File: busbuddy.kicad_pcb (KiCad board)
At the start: 2 copper layers, 77 x 54.5 mm, 48 parts, among them J201 GT-USB-7010ASV, J301 Conn_01x05_Pin, J302 Conn_01x10_Pin, J401 FH12A-24S-0.5SH(55), Q201 S8050, Q202 S8050, Q401 Q_NMOS_GSD, SW301 TS-1088R-02026, SW302 TS-1088R-02026, U202 CP2104, U301 ESP-12F, U501 SPX3819M5-L-3-3

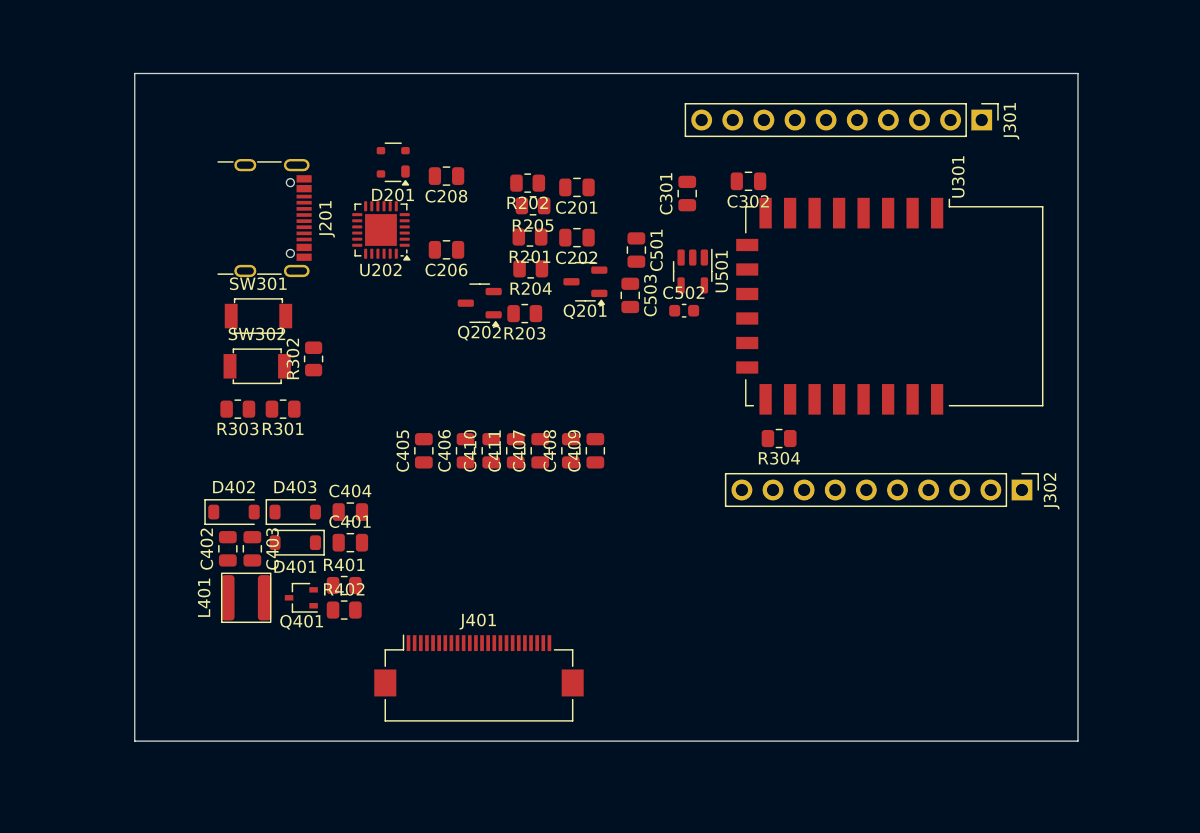
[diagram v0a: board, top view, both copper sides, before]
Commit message: Finish everything
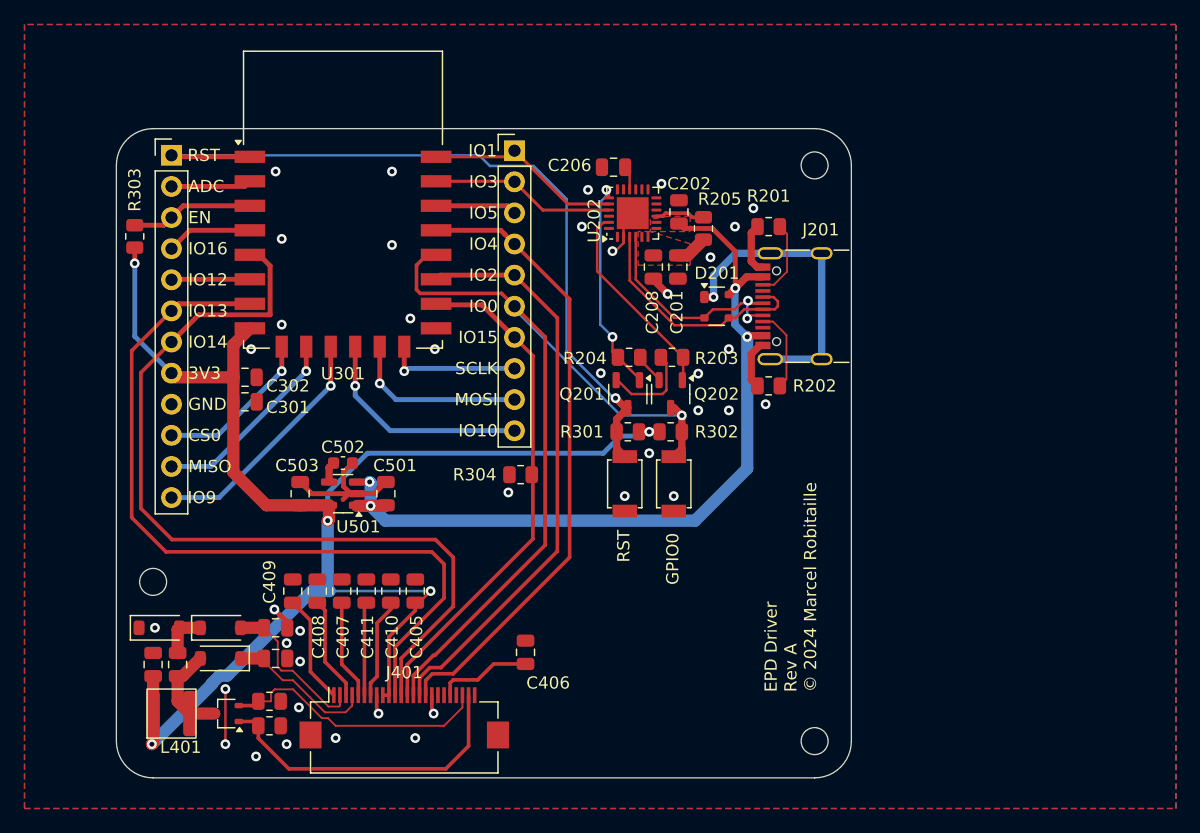
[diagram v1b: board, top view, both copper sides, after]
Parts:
- C201: value 5u -> 4u7
- J301: footprint Connector_PinHeader_2.54mm:PinHeader_1x10_P2.54mm_Vertical -> Connector_PinHeader_2.54mm:PinHeader_1x12_P2.54mm_Vertical
- moved J301 66.2 mm to (97.0, 55.7), turned to 0 degrees
- moved J302 49.8 mm to (125.0, 55.3), turned to 0 degrees
- moved U301 45.8 mm to (111.0, 59.3), turned to 0 degrees
- moved J201 45.5 mm to (149.0, 68.0), turned to 90 degrees
- moved C302 44.1 mm to (103.0, 73.8), turned to 0 degrees
- moved C301 39.9 mm to (103.0, 75.8), turned to 0 degrees
- moved SW302 35.3 mm to (138.0, 82.5), turned to 90 degrees
- moved U501 33.8 mm to (111.0, 83.3), turned to 180 degrees
- moved SW301 32.9 mm to (134.0, 82.5), turned to 90 degrees
- moved C503 31.4 mm to (107.5, 83.3), turned to 90 degrees
- moved C502 30.5 mm to (111.0, 80.8), turned to 180 degrees
- moved R302 29.8 mm to (137.8, 78.2), turned to 0 degrees
- moved D201 28.9 mm to (141.5, 68.0), turned to 0 degrees
- moved C501 28.5 mm to (114.5, 83.3), turned to 90 degrees
- moved R301 28.2 mm to (134.2, 78.2), turned to 0 degrees
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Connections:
- net Net-(D201-A) renamed /USB/SHIELD
- net Net-(J201-CC1) renamed /USB/CC1
- net Net-(J201-CC2) renamed /USB/CC2
- net Net-(U202-VPP) renamed /USB/VPP
- net Net-(U202-~{RST}) renamed /USB/CP2104_~{RST}
- net Net-(U501-BP) renamed /LDO/BYP
- D201 pad 2: /USB/D+ -> /USB/D-
- D201 pad 3: /USB/D- -> /USB/D+
- J301 pad 10: GND -> /MCU/CS0
- J301 pad 5: /EPD/SPI.SCLK -> /MCU/GPIO12
- J301 pad 6: /MCU/GPIO12 -> /EPD/SPI.MOSI
- J301 pad 7: /EPD/SPI.MOSI -> /EPD/SPI.SCLK
- J301 pad 8: /MCU/GPIO9 -> /EPD/3V3
- J301 pad 9: /EPD/3V3 -> GND
- J302 pad 1: /MCU/GPIO5 -> /MCU/TXD
- J302 pad 10: /MCU/SCLK -> /MCU/GPIO10
- J302 pad 2: /EPD/EPD_BUSY -> /MCU/RXD
- J302 pad 3: /EPD/EPD_D/C -> /MCU/GPIO5
- J302 pad 4: /EPD/EPD_RST -> /EPD/EPD_BUSY
- J302 pad 5: /EPD/SPI.~{CS} -> /EPD/EPD_RST
- J302 pad 6: /MCU/GPIO10 -> /EPD/EPD_D/C
- J302 pad 7: /MCU/CS0 -> /EPD/SPI.~{CS}
- J302 pad 8: /MCU/MISO -> /MCU/SCLK
- J401 pad 1: unconnected-(J401-NC-Pad1) -> /EPD/VCOM
- J401 pad 10: /EPD/EPD_RST -> /EPD/3V3
- J401 pad 11: /EPD/EPD_D/C -> /EPD/SPI.MOSI
- J401 pad 12: /EPD/SPI.~{CS} -> /EPD/SPI.SCLK
- J401 pad 13: /EPD/SPI.SCLK -> /EPD/SPI.~{CS}
- J401 pad 14: /EPD/SPI.MOSI -> /EPD/EPD_D/C
- J401 pad 15: /EPD/3V3 -> /EPD/EPD_RST
- J401 pad 16: /EPD/3V3 -> /EPD/EPD_BUSY
- J401 pad 18: /EPD/VDD -> unconnected-(J401-TSDA-Pad18)
- J401 pad 19: /EPD/VPP -> unconnected-(J401-TSCL-Pad19)
- J401 pad 2: /EPD/GDR -> /EPD/PREVGL
- J401 pad 20: /EPD/VSH1 -> /EPD/VSH2
- J401 pad 21: /EPD/PREVGH -> unconnected-(J401-NC-Pad21)
- J401 pad 22: /EPD/VSL -> /EPD/RESE
- J401 pad 23: /EPD/PREVGL -> /EPD/GDR
- J401 pad 24: /EPD/VCOM -> unconnected-(J401-NC-Pad24)
- J401 pad 3: /EPD/RESE -> /EPD/VSL
- J401 pad 4: unconnected-(J401-NC-Pad4) -> /EPD/PREVGH
- J401 pad 5: /EPD/VSH2 -> /EPD/VSH1
- J401 pad 6: unconnected-(J401-TSCL-Pad6) -> /EPD/VPP
- J401 pad 7: unconnected-(J401-TSDA-Pad7) -> /EPD/VDD
- J401 pad 9: /EPD/EPD_BUSY -> /EPD/3V3
- U202 pad 20: /MCU/RXD -> /MCU/TXD
- U202 pad 21: /MCU/TXD -> /MCU/RXD
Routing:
- net /EPD/3V3: track 0.00 -> 121.3 mm, vias 0 -> 5
- net /EPD/EPD_D/C: track 0.00 -> 71.8 mm, vias 0 -> 1
- net /EPD/SPI.SCLK: track 0.00 -> 69.8 mm
- net /USB/5V: track 0.00 -> 67.0 mm, vias 0 -> 4
- net /EPD/SPI.MOSI: track 0.00 -> 64.3 mm
- net /MCU/~{RST}: track 0.00 -> 64.1 mm, vias 0 -> 1
- net /EPD/EPD_BUSY: track 0.00 -> 52.6 mm
- net /EPD/EPD_RST: track 0.00 -> 47.5 mm
- net /EPD/SPI.~{CS}: track 0.00 -> 41.6 mm
- net GND: track 0.00 -> 35.7 mm, vias 0 -> 40
- net /EPD/GDR: track 0.00 -> 25.9 mm
- net /USB/SHIELD: track 0.00 -> 24.9 mm, vias 0 -> 1
- net /EPD/RESE: track 0.00 -> 22.0 mm
- net /MCU/GPIO9: track 0.00 -> 20.0 mm, vias 0 -> 1
- net /USB/D-: track 0.00 -> 19.8 mm, vias 0 -> 2
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- added copper zone on F.Cu, net /USB/5V
- added copper zone on F.Cu, net /USB/VIO
- added copper zone on B.Cu, net GND
- added copper zone on F.Cu, net GND
- added copper zone on In1.Cu, net GND
- added copper zone on In2.Cu, net GND
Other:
- board size 77 x 54.5 mm -> 60 x 53 mm
- copper layers 2 -> 4
- board text added: "3V3"
- board text added: "ADC"
- board text added: "CS0"
- board text added: "EN"
- board text added: "EPD Driver Rev A © 2024 Marcel Robitaille"
- board text added: "GND"
- board text added: "GPIO0"
- board text added: "IO0"
- board text added: "IO1"
- board text added: "IO10"
- board text added: "IO12"
- board text added: "IO13"
- board text added: "IO14"
- board text added: "IO15"
- board text added: "IO16"
- board text added: "IO2"
- board text added: "IO3"
- board text added: "IO4"
- board text added: "IO5"
- board text added: "IO9"
- board text added: "MISO"
- board text added: "MOSI"
- board text added: "RST"
- board text added: "SCLK"
